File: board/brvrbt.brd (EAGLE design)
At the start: 160 x 100 mm, 9 parts

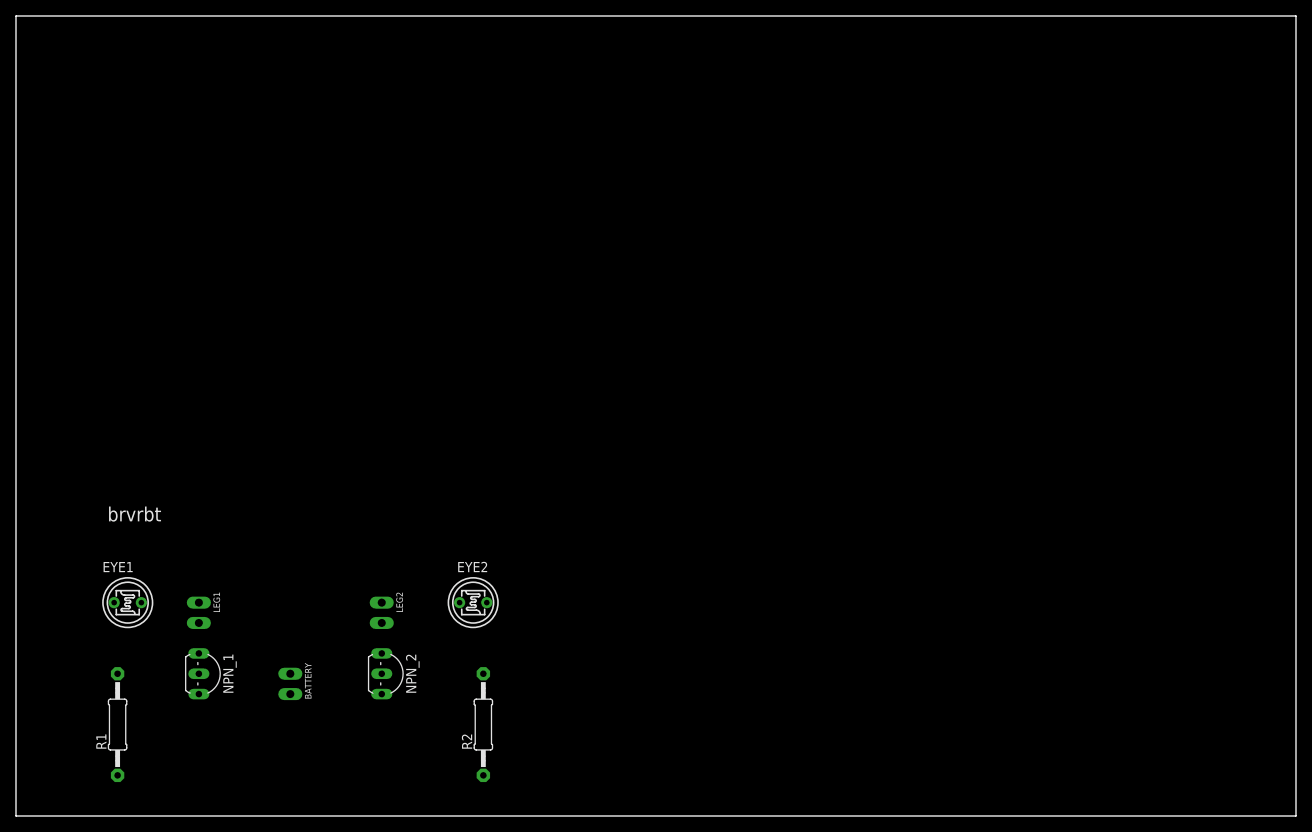
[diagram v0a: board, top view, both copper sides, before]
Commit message: layout
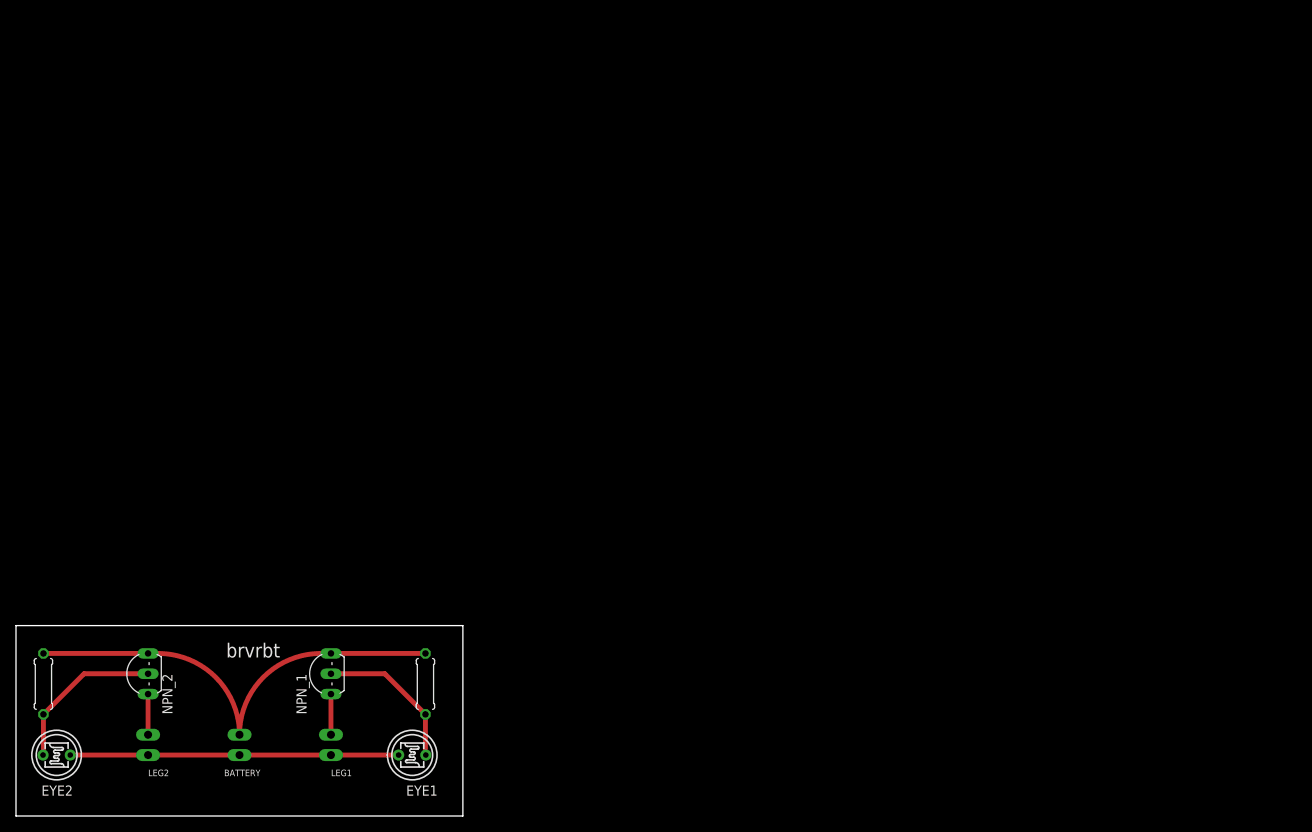
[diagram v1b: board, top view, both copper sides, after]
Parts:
- R1, R2: device adafruit:0207/12 -> adafruit:0207/7
- moved EYE2 55.4 mm to (5.08, 7.62), turned to 0 degrees
- moved R2 55.2 mm to (3.43, 16.5), turned to 270 degrees
- moved EYE1 40.3 mm to (49.5, 7.62), turned to 180 degrees
- moved R1 38.8 mm to (51.2, 16.5), turned to 270 degrees
- moved LEG2 33.6 mm to (16.5, 8.89), turned to 90 degrees
- moved NPN_2 31.8 mm to (15.2, 17.8), turned to 90 degrees
- moved LEG1 23.3 mm to (39.4, 8.89), turned to 90 degrees
- moved NPN_1 14.0 mm to (38.1, 17.8), turned to 90 degrees
- moved BATTERY 9.92 mm to (27.9, 8.89), turned to 90 degrees
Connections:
- net AGND renamed GND
- net N$1 renamed BASE_2
- net N$2 renamed COLLECTOR_2
- net N$3 renamed BASE_1
- net N$4 renamed COLLECTOR_1
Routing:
- net GND: track 0.00 -> 56.2 mm
- net VCC: track 0.00 -> 41.4 mm
- net BASE_1: track 0.00 -> 20.3 mm
- net BASE_2: track 0.00 -> 19.0 mm
- net COLLECTOR_2: track 0.00 -> 5.08 mm
- net COLLECTOR_1: track 0.00 -> 5.08 mm
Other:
- board size 160 x 100 mm -> 55.9 x 23.8 mm
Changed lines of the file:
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@@
 <board>
 <plain>
-<wire x1="0" y1="0" x2="160" y2="0" width="0" layer="20"/>
-<wire x1="160" y1="0" x2="160" y2="100" width="0" layer="20"/>
-<wire x1="160" y1="100" x2="0" y2="100" width="0" layer="20"/>
-<wire x1="0" y1="100" x2="0" y2="0" width="0" layer="20"/>
-<text x="11.43" y="36.83" size="1.778" layer="21">brvrbt</text>
+<wire x1="0" y1="0" x2="55.86" y2="0" width="0" layer="20"/>
+<wire x1="55.86" y1="0" x2="55.86" y2="23.8" width="0" layer="20"/>
+<wire x1="55.86" y1="23.8" x2="0" y2="23.8" width="0" layer="20"/>
+<wire x1="0" y1="23.8" x2="0" y2="0" width="0" layer="20"/>
+<text x="33.02" y="21.59" size="1.778" layer="21" rot="R180">brvrbt</text>
 </plain>
 <attributes>
@@
 </autorouter>
 <elements>
-<element name="R1" library="adafruit" package="0207/12" value="300Ω" x="12.7" y="11.43" smashed="yes" rot="R90">
-<attribute name="NAME" x="11.303" y="8.255" size="1.27" layer="25" ratio="10" rot="R90"/>
-<attribute name="VALUE" x="13.3858" y="9.144" size="1.27" layer="27" ratio="10" rot="R90"/>
-</element>
-<element name="NPN_1" library="transistor" library_urn="urn:adsk.eagle:library:402" package="TO92-EBC" value="" x="24.13" y="17.78" smashed="yes" rot="R270">
-<attribute name="NAME" x="25.908" y="20.32" size="1.27" layer="25" ratio="10" rot="R270"/>
-<attribute name="VALUE" x="19.558" y="20.32" size="1.27" layer="27" ratio="10" rot="R270"/>
-</element>
-<element name="EYE1" library="photo-elements" library_urn="urn:adsk.eagle:library:323" package="T0-46-A10XX" value="A1050_09" x="13.97" y="26.67" smashed="yes">
-<attribute name="NAME" x="10.795" y="30.48" size="1.27" layer="25"/>
-</element>
-<element name="LEG1" library="microbuilder" package="1X02_OVAL" value="" x="22.86" y="25.4" rot="R270"/>
-<element name="BATTERY" library="microbuilder" package="1X02_OVAL" value="" x="34.29" y="16.51" rot="R270"/>
-<element name="R2" library="adafruit" package="0207/12" value="300Ω" x="58.42" y="11.43" smashed="yes" rot="R90">
-<attribute name="NAME" x="57.023" y="8.255" size="1.27" layer="25" ratio="10" rot="R90"/>
-<attribute name="VALUE" x="59.1058" y="9.144" size="1.27" layer="27" ratio="10" rot="R90"/>
-</element>
-<element name="NPN_2" library="transistor" library_urn="urn:adsk.eagle:library:402" package="TO92-EBC" value="" x="46.99" y="17.78" smashed="yes" rot="R270">
-<attribute name="NAME" x="48.768" y="20.32" size="1.27" layer="25" ratio="10" rot="R270"/>
-<attribute name="VALUE" x="42.418" y="20.32" size="1.27" layer="27" ratio="10" rot="R270"/>
-</element>
-<element name="EYE2" library="photo-elements" library_urn="urn:adsk.eagle:library:323" package="T0-46-A10XX" value="A1050_09" x="57.15" y="26.67" smashed="yes" rot="R180">
-<attribute name="NAME" x="59.055" y="31.75" size="1.27" layer="25" rot="R180"/>
-</element>
-<element name="LEG2" library="microbuilder" package="1X02_OVAL" value="" x="45.72" y="25.4" rot="R270"/>
+<element name="R1" library="adafruit" package="0207/7" value="300Ω" x="51.181" y="16.51" smashed="yes" rot="R270">
+<attribute name="VALUE" x="50.4952" y="18.796" size="1.27" layer="27" ratio="10" rot="R270"/>
+</element>
+<element name="NPN_1" library="transistor" library_urn="urn:adsk.eagle:library:402" package="TO92-EBC" value="" x="38.1" y="17.78" smashed="yes" rot="R90">
+<attribute name="NAME" x="36.321996875" y="12.699996875" size="1.27" layer="25" ratio="10" rot="R90"/>
+<attribute name="VALUE" x="42.672" y="15.24" size="1.27" layer="27" ratio="10" rot="R90"/>
+</element>
+<element name="EYE1" library="photo-elements" library_urn="urn:adsk.eagle:library:323" package="T0-46-A10XX" value="A1050_09" x="49.53" y="7.62" smashed="yes" rot="R180">
+<attribute name="NAME" x="52.705" y="3.81" size="1.27" layer="25" rot="R180"/>
+</element>
+<element name="LEG1" library="microbuilder" package="1X02_OVAL" value="" x="39.37" y="8.89" smashed="yes" rot="R90">
+<attribute name="NAME" x="41.9862" y="5.7912" size="0.8128" layer="25" ratio="18" rot="R180"/>
+<attribute name="VALUE" x="42.545" y="6.35" size="0.4064" layer="27" ratio="10" rot="R90"/>
+</element>
+<element name="BATTERY" library="microbuilder" package="1X02_OVAL" value="" x="27.94" y="8.89" smashed="yes" rot="R90">
+<attribute name="NAME" x="30.5562" y="5.7912" size="0.8128" layer="25" ratio="18" rot="R180"/>
+<attribute name="VALUE" x="31.115" y="6.35" size="0.4064" layer="27" ratio="10" rot="R90"/>
+</element>
+<element name="R2" library="adafruit" package="0207/7" value="300Ω" x="3.429" y="16.51" smashed="yes" rot="R270">
+<attribute name="VALUE" x="2.7432" y="18.796" size="1.27" layer="27" ratio="10" rot="R270"/>
+</element>
+<element name="NPN_2" library="transistor" library_urn="urn:adsk.eagle:library:402" package="TO92-EBC" value="" x="15.24" y="17.78" smashed="yes" rot="R90">
+<attribute name="NAME" x="18.288003125" y="17.78" size="1.27" layer="25" ratio="10" rot="R270"/>
+<attribute name="VALUE" x="19.812" y="15.24" size="1.27" layer="27" ratio="10" rot="R90"/>
+</element>
+<element name="EYE2" library="photo-elements" library_urn="urn:adsk.eagle:library:323" package="T0-46-A10XX" value="A1050_09" x="5.08" y="7.62" smashed="yes">
+<attribute name="NAME" x="3.175" y="2.54" size="1.27" layer="25"/>
+</element>
+<element name="LEG2" library="microbuilder" package="1X02_OVAL" value="" x="16.51" y="8.89" smashed="yes" rot="R90">
+<attribute name="NAME" x="19.1262" y="5.7912" size="0.8128" layer="25" ratio="18" rot="R180"/>
+<attribute name="VALUE" x="19.685" y="6.35" size="0.4064" layer="27" ratio="10" rot="R90"/>
+</element>
 </elements>
 <signals>
-<signal name="AGND">
+<signal name="GND">
 <contactref element="BATTERY" pad="2"/>
 <contactref element="R1" pad="1"/>
@@
 <contactref element="R2" pad="1"/>
 <contactref element="NPN_2" pad="C"/>
-<wire x1="45.72" y1="15.24" x2="58.42" y2="5.08" width="0" layer="19" extent="1-1"/>
-<wire x1="34.29" y1="15.24" x2="45.72" y2="15.24" width="0" layer="19" extent="1-1"/>
-<wire x1="22.86" y1="15.24" x2="34.29" y2="15.24" width="0" layer="19" extent="1-1"/>
-<wire x1="12.7" y1="5.08" x2="22.86" y2="15.24" width="0" layer="19" extent="1-1"/>
-</signal>
-<signal name="N$1">
+<wire x1="3.429" y1="20.32" x2="16.51" y2="20.32" width="0.6096" layer="1"/>
+<wire x1="51.181" y1="20.32" x2="39.37" y2="20.32" width="0.6096" layer="1"/>
+<wire x1="16.51" y1="20.32" x2="17.78" y2="20.32" width="0.6096" layer="1"/>
+<wire x1="27.94" y1="10.16" x2="17.78" y2="20.32" width="0.6096" layer="1" curve="90"/>
+<wire x1="39.37" y1="20.32" x2="38.1" y2="20.32" width="0.6096" layer="1"/>
+<wire x1="38.1" y1="20.32" x2="27.94" y2="10.16" width="0.6096" layer="1" curve="90"/>
+</signal>
+<signal name="BASE_2">
 <contactref element="R1" pad="2"/>
 <contactref element="EYE1" pad="1"/>
 <contactref element="NPN_1" pad="B"/>
-<wire x1="12.7" y1="17.78" x2="22.86" y2="17.78" width="0" layer="19" extent="1-1"/>
-<wire x1="12.27" y1="26.67" x2="12.7" y2="17.78" width="0" layer="19" extent="1-1"/>
+<wire x1="39.37" y1="17.78" x2="46.101" y2="17.78" width="0.6096" layer="1"/>
+<wire x1="46.101" y1="17.78" x2="51.181" y2="12.7" width="0.6096" layer="1"/>
+<wire x1="51.181" y1="12.7" x2="51.181" y2="7.669" width="0.6096" layer="1"/>
+<wire x1="51.181" y1="7.669" x2="51.23" y2="7.62" width="0.6096" layer="1"/>
 </signal>
 <signal name="VCC">
@@
 <contactref element="EYE2" pad="2"/>
 <contactref element="LEG2" pad="1"/>
-<wire x1="45.72" y1="26.67" x2="55.45" y2="26.67" width="0" layer="19" extent="1-1"/>
-<wire x1="34.29" y1="17.78" x2="45.72" y2="26.67" width="0" layer="19" extent="1-1"/>
-<wire x1="22.86" y1="26.67" x2="34.29" y2="17.78" width="0" layer="19" extent="1-1"/>
-<wire x1="15.67" y1="26.67" x2="22.86" y2="26.67" width="0" layer="19" extent="1-1"/>
-</signal>
-<signal name="N$2">
+<wire x1="47.83" y1="7.62" x2="39.37" y2="7.62" width="0.6096" layer="1"/>
+<wire x1="16.187025" y1="7.62" x2="6.78" y2="7.62" width="0.6096" layer="1"/>
+<wire x1="16.187025" y1="7.62" x2="16.51" y2="7.62" width="0.4064" layer="1"/>
+<wire x1="39.37" y1="7.62" x2="27.94" y2="7.62" width="0.6096" layer="1"/>
+<wire x1="27.94" y1="7.62" x2="16.187025" y2="7.62" width="0.6096" layer="1"/>
+</signal>
+<signal name="COLLECTOR_2">
 <contactref element="LEG1" pad="2"/>
 <contactref element="NPN_1" pad="E"/>
-<wire x1="22.86" y1="20.32" x2="22.86" y2="24.13" width="0" layer="19" extent="1-1"/>
-</signal>
-<signal name="N$3">
+<wire x1="39.37" y1="15.24" x2="39.37" y2="10.16" width="0.6096" layer="1"/>
+</signal>
+<signal name="BASE_1">
 <contactref element="R2" pad="2"/>
 <contactref element="EYE2" pad="1"/>
 <contactref element="NPN_2" pad="B"/>
-<wire x1="58.42" y1="17.78" x2="58.85" y2="26.67" width="0" layer="19" extent="1-1"/>
-<wire x1="45.72" y1="17.78" x2="58.42" y2="17.78" width="0" layer="19" extent="1-1"/>
-</signal>
-<signal name="N$4">
+<wire x1="16.51" y1="17.78" x2="8.509" y2="17.78" width="0.6096" layer="1"/>
+<wire x1="8.509" y1="17.78" x2="3.429" y2="12.7" width="0.6096" layer="1"/>
+<wire x1="3.429" y1="12.7" x2="3.429" y2="7.669" width="0.6096" layer="1"/>
+<wire x1="3.429" y1="7.669" x2="3.38" y2="7.62" width="0.6096" layer="1"/>
+</signal>
+<signal name="COLLECTOR_1">
 <contactref element="LEG2" pad="2"/>
 <contactref element="NPN_2" pad="E"/>
-<wire x1="45.72" y1="20.32" x2="45.72" y2="24.13" width="0" layer="19" extent="1-1"/>
+<wire x1="16.51" y1="10.16" x2="16.51" y2="15.24" width="0.6096" layer="1"/>
 </signal>
 </signals>
